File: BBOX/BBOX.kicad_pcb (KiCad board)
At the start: 2 copper layers, 47 x 42.7 mm, 20 parts, among them J1 BBOX, J10 LED, J2 WJ127-5.0-2P, J3 Servo2, J7 IR_LEDs, J9 Servo1, Q1 IRLML2502PBF, U2 AP2210N-3.3TRG1, U4 PCA9685PW, U5 PCA9306

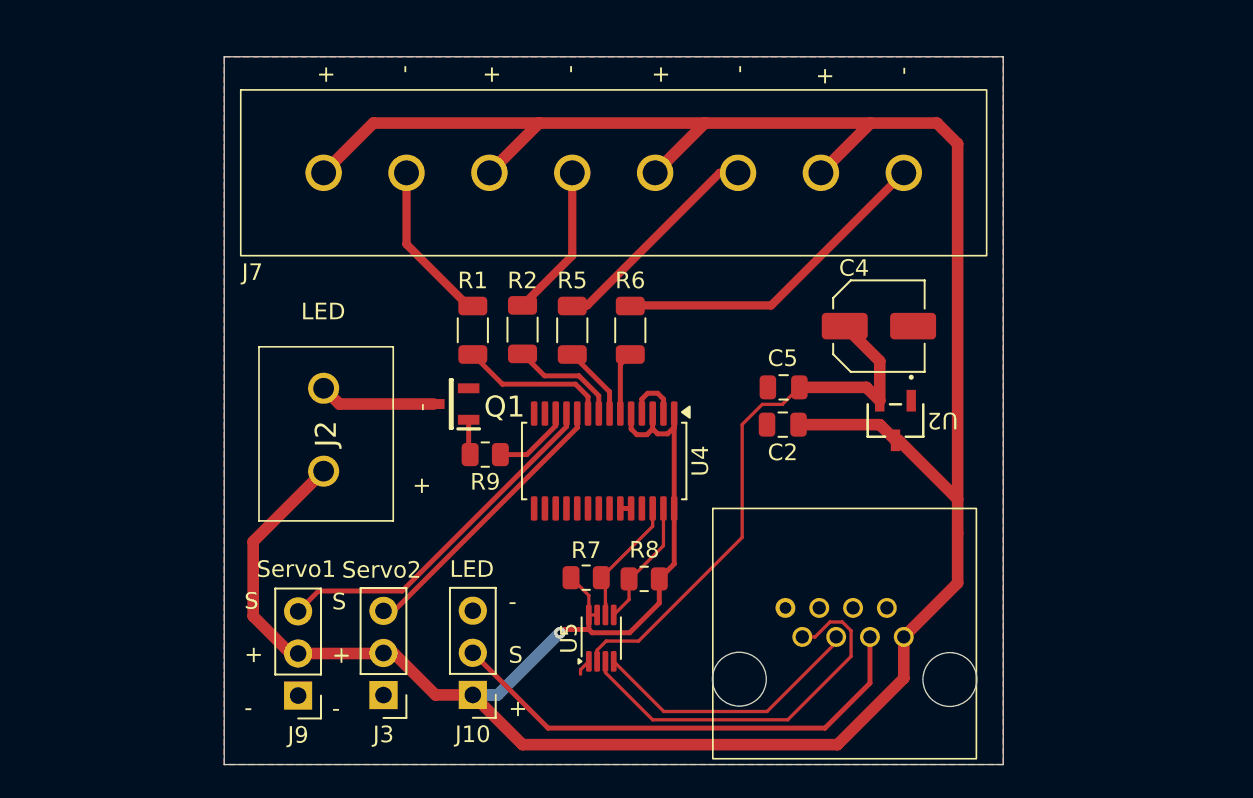
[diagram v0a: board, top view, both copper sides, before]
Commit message: v1.0
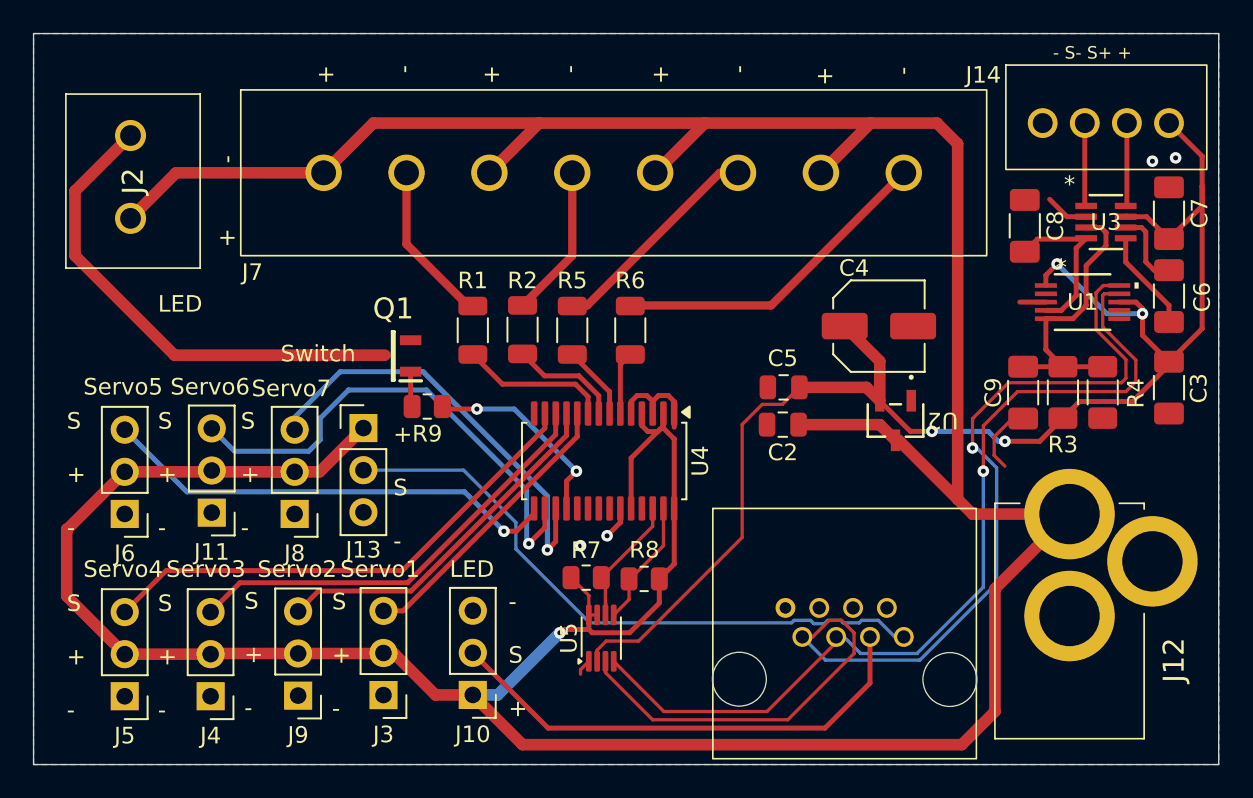
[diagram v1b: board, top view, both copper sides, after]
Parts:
- added C3: 0.1u, Capacitor_SMD:C_1206_3216Metric_Pad1.33x1.80mm_HandSolder, F.Cu at (197.0, 85.0)
- added C6: 1.3n, Capacitor_SMD:C_1206_3216Metric_Pad1.33x1.80mm_HandSolder, F.Cu at (197.0, 79.4)
- added C7: 0.1u, Capacitor_SMD:C_1206_3216Metric_Pad1.33x1.80mm_HandSolder, F.Cu at (197.0, 74.4)
- added C8: 39n, Capacitor_SMD:C_1206_3216Metric_Pad1.33x1.80mm_HandSolder, F.Cu at (188.3, 75.2)
- added C9: 0.1u, Capacitor_SMD:C_1206_3216Metric_Pad1.33x1.80mm_HandSolder, F.Cu at (188.2, 85.3)
- added J11: Servo6, Connector_PinHeader_2.54mm:PinHeader_1x03_P2.54mm_Vertical, F.Cu at (139.2, 92.5)
- added J12: FC68148, FC68148:FC68148, F.Cu at (191.0, 92.6)
- added J13: SWITCH, Connector_PinHeader_2.54mm:PinHeader_1x03_P2.54mm_Vertical, F.Cu at (148.4, 87.4)
- added J14: Scale, JL308-25404G01:JL308-25404G01, F.Cu at (187.4, 72.0)
- added J4: Servo3, Connector_PinHeader_2.54mm:PinHeader_1x03_P2.54mm_Vertical, F.Cu at (139.2, 103.6)
- added J5: Servo4, Connector_PinHeader_2.54mm:PinHeader_1x03_P2.54mm_Vertical, F.Cu at (134.0, 103.6)
- added J6: Servo5, Connector_PinHeader_2.54mm:PinHeader_1x03_P2.54mm_Vertical, F.Cu at (134.0, 92.6)
- added J8: Servo7, Connector_PinHeader_2.54mm:PinHeader_1x03_P2.54mm_Vertical, F.Cu at (144.2, 92.6)
- added R3: 100k, Resistor_SMD:R_1206_3216Metric_Pad1.30x1.75mm_HandSolder, F.Cu at (190.6, 85.2)
- added R4: 100k, Resistor_SMD:R_1206_3216Metric_Pad1.30x1.75mm_HandSolder, F.Cu at (193.0, 85.2)
- added U1: ADS1114IDGS, ADS1114IDGST:DGS10, F.Cu at (191.8, 79.8)
- added U3: AD8293G80ARJZ-R7, AD8293G80ARJZ-R7:RJ_8_ADI, F.Cu at (193.2, 75.0)
- J3: value Servo2 -> Servo1
- J9: value Servo1 -> Servo2
- moved J2 19.2 mm to (134.3, 74.8)
- moved Q1 4.55 mm to (150.2, 83.0)
- moved R9 4.55 mm to (152.2, 86.1)
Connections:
- J1 pad 8: +VDC -> SWITCH
- R9 pad 1: STRIP_PWM -> Net-(U4-LED11)
- U4 pad 1: +VDC -> GND
- U4 pad 12: STRIP_PWM -> Net-(J4-Pin_3)
- U4 pad 13: unconnected-(U4-LED7-Pad13) -> Net-(J5-Pin_3)
- U4 pad 15: unconnected-(U4-LED8-Pad15) -> Net-(J6-Pin_3)
- U4 pad 16: unconnected-(U4-LED9-Pad16) -> Net-(J11-Pin_3)
- U4 pad 17: unconnected-(U4-LED10-Pad17) -> Net-(J8-Pin_3)
- U4 pad 18: unconnected-(U4-LED11-Pad18) -> Net-(U4-LED11)
- U4 pad 2: GND -> +VDC
- U4 pad 24: GND -> +VDC
- U4 pad 3: +VDC -> GND
- U4 pad 4: GND -> +VDC
- U4 pad 5: +VDC -> GND
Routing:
- net +3.3VA: track 34.0 -> 91.3 mm, vias 0 -> 4
- net +VDC: track 187.9 -> 244.0 mm
- net I2C_SCL: track 23.3 -> 66.3 mm, vias 0 -> 1
- net SWITCH: track 0.00 -> 38.1 mm
- net I2C_SDA: track 16.7 -> 54.8 mm, vias 0 -> 1
- net Net-(J5-Pin_3): track 0.00 -> 30.8 mm
- net Net-(J11-Pin_3): track 0.00 -> 30.4 mm, vias 0 -> 1
- net Net-(J6-Pin_3): track 0.00 -> 28.0 mm, vias 0 -> 1
- net Net-(J4-Pin_3): track 0.00 -> 26.5 mm
- net Net-(J8-Pin_3): track 0.00 -> 26.2 mm, vias 0 -> 1
- net Net-(Q1-D): track 7.04 -> 29.8 mm
- net Net-(U1-AIN1): track 0.00 -> 17.1 mm
- net GND: track 4.97 -> 17.6 mm, vias 0 -> 4
- net Net-(U4-LED11): track 0.00 -> 12.2 mm, vias 0 -> 2
- net Net-(U1-AIN0): track 0.00 -> 9.93 mm
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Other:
- board size 47 x 42.7 mm -> 71.5 x 44.1 mm
- board text added: "*"
- board text added: "+ S -"
- board text added: "- S- S+ +"
- board text added: "Servo3"
- board text added: "Servo4"
- board text added: "Servo5"
- board text added: "Servo6"
- board text added: "Servo7"
- board text added: "Switch"
